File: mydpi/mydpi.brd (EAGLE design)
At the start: 41 x 20 mm, 34 parts, among them Q1 DMN3404L, U1 MEGA32U4-MU, U2 RT9193-33GB, Y1 830069392

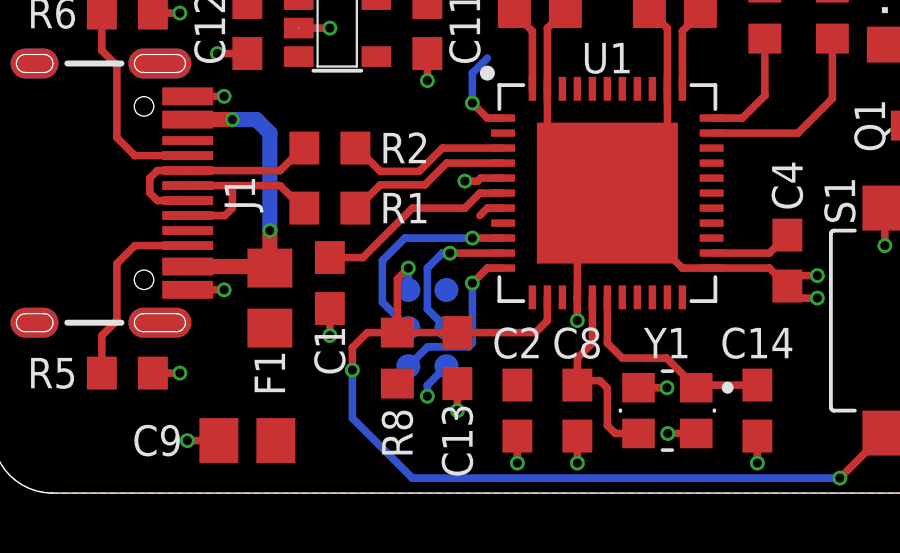
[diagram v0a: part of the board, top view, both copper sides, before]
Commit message: Bugfixes in used libraries
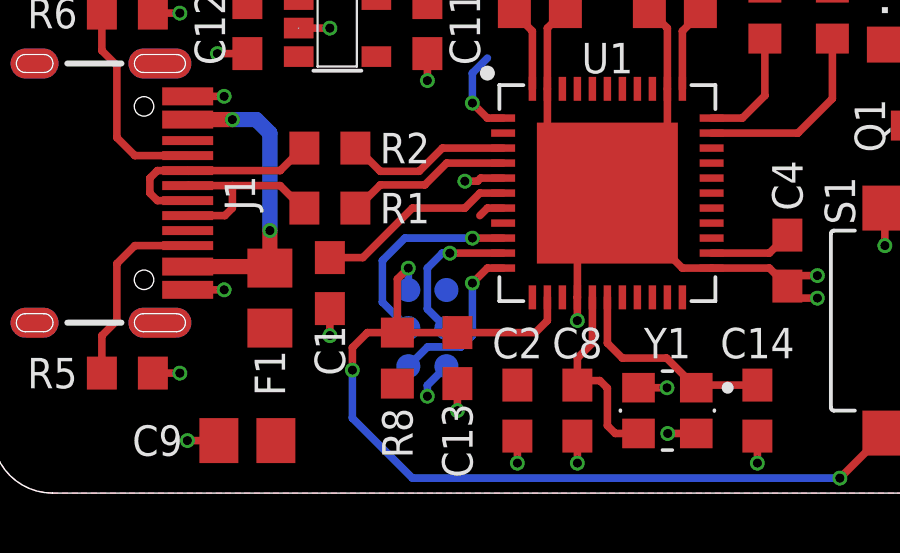
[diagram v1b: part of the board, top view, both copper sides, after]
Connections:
- removed net MEDBG_UPDI: DBG1.3, R4.2
- new net N$3: R4.2
- new net UDPI: DBG1.3
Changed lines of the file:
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@@
 </attributes>
 <variantdefs>
+<variantdef name="BOM"/>
 </variantdefs>
 <classes>
@@
 <attribute name="VOLTAGE" value="75V" x="25.75" y="16" size="1.778" layer="27" rot="R90" display="off"/>
 </element>
-<element name="ICSP1" library="zaan-Connectors" library_urn="urn:adsk.eagle:library:16759010" package="AVRISP-1.27-SMD" value="AVR-ISP-SMD" x="14.5" y="5.5" smashed="yes" rot="MR180">
+<element name="ICSP1" library="zaan-Connectors" library_urn="urn:adsk.eagle:library:16759010" package="AVRISP-1.27-SMD" package3d_urn="urn:adsk.eagle:package:17075154/1" value="AVR-ISP-SMD" x="14.5" y="5.5" smashed="yes" rot="MR180">
 <attribute name="NAME" x="17" y="5.5" size="1.016" layer="26" font="vector" ratio="15" rot="MR90" align="center"/>
 </element>
@@
 </element>
 <element name="Y1" library="zaan-Electromechanical" library_urn="urn:adsk.eagle:library:16759157" package="WE-XTAL_CFPX-218" package3d_urn="urn:adsk.eagle:package:16759170/1" value="830069392" x="22.5" y="2.75" smashed="yes" rot="R180">
+<attribute name="DESCRIPTION" value="Crystal" x="22.5" y="2.75" size="1.778" layer="27" rot="R180" display="off"/>
+<attribute name="MF" value="Wurth Electronics" x="22.5" y="2.75" size="1.778" layer="27" rot="R180" display="off"/>
+<attribute name="MPN" value="830069392" x="22.5" y="2.75" size="1.778" layer="27" rot="R180" display="off"/>
 <attribute name="NAME" x="22.5" y="5" size="1.016" layer="25" font="vector" ratio="15" align="center"/>
+<attribute name="PACKAGE" value="2520" x="22.5" y="2.75" size="1.778" layer="27" rot="R180" display="off"/>
 <attribute name="VALUE" x="22.5" y="5.25" size="1.016" layer="27" font="vector" ratio="15" rot="R180" align="center"/>
 </element>
@@
 </element>
 <element name="S1" library="zaan-Electromechanical" library_urn="urn:adsk.eagle:library:16759157" package="SPST-6X3.6" package3d_urn="urn:adsk.eagle:package:16760026/2" value="TS-1101-C-W" x="29.75" y="5.75" smashed="yes" rot="R270">
+<attribute name="DESCRIPTION" value="Tactile Button" x="29.75" y="5.75" size="1.778" layer="27" rot="R270" display="off"/>
+<attribute name="MF" value="Korean Hroparts Elec" x="29.75" y="5.75" size="1.778" layer="27" rot="R270" display="off"/>
+<attribute name="MPN" value="K2-1107ST-A4SW-06" x="29.75" y="5.75" size="1.778" layer="27" rot="R270" display="off"/>
 <attribute name="NAME" x="28.25" y="9.75" size="1.016" layer="25" font="vector" ratio="15" rot="R270" align="center"/>
+<attribute name="PACKAGE" value="6.1X3.6X2.5" x="29.75" y="5.75" size="1.778" layer="27" rot="R270" display="off"/>
 <attribute name="VALUE" x="27.25" y="5.75" size="1.016" layer="27" font="vector" ratio="15" rot="R270" align="center"/>
 </element>
@@
 <attribute name="MPN" value="MF-PSMF035X-2" x="9.25" y="6.5" size="1.778" layer="27" rot="R270" display="off"/>
 <attribute name="NAME" x="9.25" y="4" size="1.016" layer="25" font="vector" ratio="15" rot="R270" align="center"/>
-<attribute name="PACKAGE" value="0805" x="9.25" y="6.5" size="1.778" layer="27" rot="R270" display="off"/>
+<attribute name="PACKAGE" value="2012" x="9.25" y="6.5" size="1.778" layer="27" rot="R270" display="off"/>
 <attribute name="VALUE" x="5.75" y="6.5" size="1.016" layer="27" font="vector" ratio="15" rot="R270" align="center"/>
 </element>
@@
 <wire x1="8.5" y1="14.65" x2="7.5" y2="14.65" width="0.254" layer="1"/>
 <via x="7.5" y="14.65" extent="1-16" drill="0.3"/>
+<wire x1="33.25" y1="7.25" x2="38.77" y2="11.905" width="0" layer="19" extent="1-1"/>
+<wire x1="29.75" y1="8.25" x2="32.25" y2="7.25" width="0" layer="19" extent="1-1"/>
+<wire x1="27.5" y1="7.25" x2="29.75" y2="8.25" width="0" layer="19" extent="1-1"/>
+<wire x1="20.5" y1="10" x2="22.75" y2="7.75" width="0" layer="19" extent="1-1"/>
+<wire x1="22.5" y1="12" x2="20.5" y2="10" width="0" layer="19" extent="1-1"/>
+<wire x1="19.5" y1="17" x2="21.5" y2="17" width="0" layer="19" extent="1-1"/>
+<wire x1="17.025" y1="10.5" x2="18.5" y2="12" width="0" layer="19" extent="1-1"/>
+<wire x1="21.5375" y1="3.5125" x2="19.498" y2="5.75" width="0" layer="19" extent="1-1"/>
+<wire x1="22.5125" y1="1.9875" x2="22.4875" y2="3.5125" width="0" layer="19" extent="1-1"/>
+<wire x1="25.5" y1="1.9" x2="23.4625" y2="1.9875" width="0" layer="19" extent="1-1"/>
+<wire x1="19.5" y1="1.9" x2="21.5375" y2="3.5125" width="0" layer="19" extent="1-1"/>
+<wire x1="17.5" y1="1.9" x2="19.5" y2="1.9" width="0" layer="19" extent="1-1"/>
+<wire x1="15.5" y1="2.75" x2="17.5" y2="1.9" width="0" layer="19" extent="1-1"/>
+<wire x1="15.135" y1="6.77" x2="15.5" y2="3.65" width="0" layer="19" extent="1-16"/>
+<wire x1="14.5" y1="13.75" x2="15.75" y2="10.398" width="0" layer="19" extent="1-1"/>
+<wire x1="11.25" y1="15.5" x2="14.5" y2="14.65" width="0" layer="19" extent="1-1"/>
+<wire x1="8.5" y1="14.65" x2="10.21" y2="15.5" width="0" layer="19" extent="1-1"/>
+<wire x1="7.725" y1="13.225" x2="7.5" y2="14.65" width="0" layer="19" extent="1-1"/>
+<wire x1="6.25" y1="16" x2="7.5" y2="14.65" width="0" layer="19" extent="1-1"/>
+<wire x1="12.75" y1="18" x2="11.25" y2="15.5" width="0" layer="19" extent="1-1"/>
+<wire x1="11.25" y1="6.15" x2="15.135" y2="6.77" width="0" layer="19" extent="1-16"/>
+<wire x1="7.725" y1="6.775" x2="11.25" y2="6.15" width="0" layer="19" extent="1-1"/>
+<wire x1="6.25" y1="4" x2="6.51" y2="6.775" width="0" layer="19" extent="1-1"/>
+<wire x1="6.5" y1="1.75" x2="6.25" y2="4" width="0" layer="19" extent="1-1"/>
+<wire x1="1.95" y1="18.5" x2="5.35" y2="16" width="0" layer="19" extent="1-1"/>
 </signal>
 <signal name="+5V">
@@
 <wire x1="14.5" y1="3.595" x2="14.5" y2="3.23" width="0.254" layer="16"/>
 <via x="14.5" y="3.23" extent="1-16" drill="0.3"/>
-<wire x1="8.35" y1="18.5" x2="13" y2="28" width="0" layer="19" extent="1-1"/>
+<wire x1="25.75" y1="16.85" x2="29.75" y2="14.95" width="0" layer="19" extent="1-1"/>
+<wire x1="23.6" y1="16" x2="25.75" y2="16.85" width="0" layer="19" extent="1-1"/>
+<wire x1="19" y1="13.475" x2="23" y2="13.475" width="0" layer="19" extent="1-1"/>
+<wire x1="18" y1="13.475" x2="19" y2="13.475" width="0" layer="19" extent="1-1"/>
+<wire x1="17.025" y1="12" x2="18" y2="13.475" width="0" layer="19" extent="1-1"/>
+<wire x1="17.025" y1="9.5" x2="17.025" y2="12" width="0" layer="19" extent="1-1"/>
+<wire x1="19" y1="6.525" x2="17.025" y2="9.5" width="0" layer="19" extent="1-1"/>
+<wire x1="17.5" y1="3.6" x2="19" y2="6.525" width="0" layer="19" extent="1-1"/>
+<wire x1="15.135" y1="4.23" x2="17.5" y2="3.6" width="0" layer="19" extent="1-16"/>
+<wire x1="13.5" y1="3.65" x2="14.5" y2="3.23" width="0" layer="19" extent="1-1"/>
+<wire x1="9.45" y1="1.75" x2="13.5" y2="3.65" width="0" layer="19" extent="1-1"/>
+<wire x1="9.25" y1="5.5" x2="9.45" y2="1.75" width="0" layer="19" extent="1-1"/>
+<wire x1="23.975" y1="8" x2="19" y2="6.525" width="0" layer="19" extent="1-1"/>
+<wire x1="10.21" y1="16.45" x2="17.4" y2="16" width="0" layer="19" extent="1-1"/>
+<wire x1="8.5" y1="16.35" x2="10.21" y2="16.45" width="0" layer="19" extent="1-1"/>
+<wire x1="8.35" y1="18.5" x2="8.5" y2="16.35" width="0" layer="19" extent="1-1"/>
+<wire x1="13" y1="28" x2="8.35" y2="18.5" width="0" layer="19" extent="1-1"/>
 </signal>
 <signal name="N$1">
@@
 <wire x1="8" y1="10.25" x2="8" y2="9.5" width="0.254" layer="1"/>
 </signal>
-<signal name="MEDBG_UPDI">
-<contactref element="DBG1" pad="3"/>
-<contactref element="R4" pad="2"/>
-<wire x1="32.5" y1="14.9" x2="36.23" y2="10.635" width="0" layer="19" extent="1-1"/>
-</signal>
 <signal name="+3V3">
 <contactref element="SJ1" pad="1"/>
@@
 <contactref element="ICSP1" pad="1"/>
 <wire x1="13.865" y1="4.23" x2="14.508" y2="4.873" width="0.254" layer="16"/>
-<wire x1="15.873" y1="4.873" x2="16" y2="5" width="0.254" layer="16"/>
+<wire x1="15.623" y1="4.873" x2="16" y2="5.25" width="0.254" layer="16"/>
 <via x="16" y="7" extent="1-16" drill="0.3"/>
 <wire x1="16" y1="7" x2="16.5" y2="7.5" width="0.254" layer="1"/>
 <wire x1="16.5" y1="7.5" x2="17.025" y2="7.5" width="0.254" layer="1"/>
-<wire x1="14.508" y1="4.873" x2="15.873" y2="4.873" width="0.254" layer="16"/>
-<wire x1="16" y1="5" x2="16" y2="7" width="0.254" layer="16"/>
+<wire x1="14.508" y1="4.873" x2="15.623" y2="4.873" width="0.254" layer="16"/>
+<wire x1="16" y1="5.25" x2="16" y2="7" width="0.254" layer="16"/>
 </signal>
 <signal name="RST">
@@
 <wire x1="12" y1="28.5" x2="15.35" y2="18" width="0" layer="19" extent="1-16"/>
 </signal>
+<signal name="UDPI">
+<contactref element="DBG1" pad="3"/>
+</signal>
+<signal name="N$3">
+<contactref element="R4" pad="2"/>
+</signal>
 </signals>
